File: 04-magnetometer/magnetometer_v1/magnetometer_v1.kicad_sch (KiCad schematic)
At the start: 42 parts, among them IC1 STM32F072CBT6, IC2 TMAG5170A1QDGKR, IC3 TCAN1042GVDRQ1, J1 Conn_02x04_Odd_Even, J2 USB4110-GF-A, SW3 SW_SPDT, U1 SPX3819M5-L-3-3/TR, U2 NANOT100AS, U3 NANOT100AS

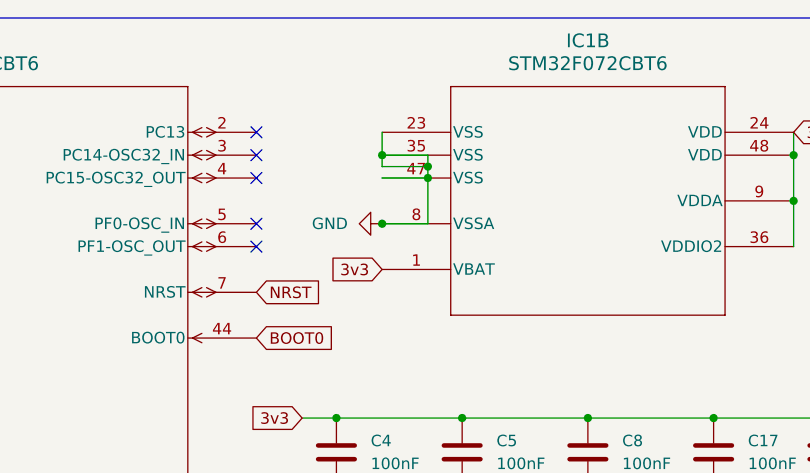
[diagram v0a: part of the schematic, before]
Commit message: made review changes
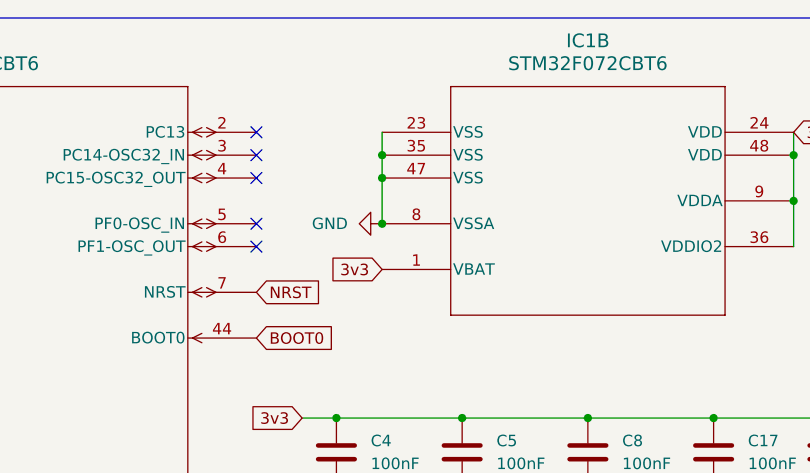
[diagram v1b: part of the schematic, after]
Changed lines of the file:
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@@
 	)
 	(junction
-		(at 114.3 33.02)
+		(at 109.22 34.29)
 		(diameter 0)
 		(color 0 0 0 0)
@@
 	)
 	(junction
-		(at 114.3 34.29)
-		(diameter 0)
-		(color 0 0 0 0)
-	)
-	(junction
 		(at 113.03 151.13)
 		(diameter 0)
@@
 	(wire
 		(pts
-			(xy 109.22 33.02) (xy 114.3 33.02)
-		)
-		(stroke
-			(width 0)
-			(type default)
-		)
-	)
-	(wire
-		(pts
 			(xy 143.51 118.11) (xy 143.51 119.38)
 		)
@@
 	(wire
 		(pts
-			(xy 114.3 33.02) (xy 114.3 34.29)
-		)
-		(stroke
-			(width 0)
-			(type default)
-		)
-	)
-	(wire
-		(pts
 			(xy 104.14 78.74) (xy 118.11 78.74)
 		)
@@
 	(wire
 		(pts
-			(xy 114.3 33.02) (xy 114.3 31.75)
-		)
-		(stroke
-			(width 0)
-			(type default)
-		)
-	)
-	(wire
-		(pts
 			(xy 251.46 118.11) (xy 248.92 118.11)
 		)
@@
 	(wire
 		(pts
-			(xy 109.22 34.29) (xy 114.3 34.29)
-		)
-		(stroke
-			(width 0)
-			(type default)
-		)
-	)
-	(wire
-		(pts
 			(xy 248.92 114.3) (xy 259.08 114.3)
 		)
@@
 	(wire
 		(pts
-			(xy 109.22 31.75) (xy 109.22 33.02)
+			(xy 109.22 31.75) (xy 109.22 34.29)
 		)
 		(stroke
@@
 	(wire
 		(pts
-			(xy 109.22 39.37) (xy 114.3 39.37)
-		)
-		(stroke
-			(width 0)
-			(type default)
-		)
-	)
-	(wire
-		(pts
 			(xy 215.9 142.24) (xy 215.9 147.32)
 		)
@@
 	(wire
 		(pts
-			(xy 114.3 34.29) (xy 114.3 39.37)
-		)
-		(stroke
-			(width 0)
-			(type default)
-		)
-	)
-	(wire
-		(pts
-			(xy 109.22 31.75) (xy 114.3 31.75)
-		)
-		(stroke
+			(xy 109.22 34.29) (xy 109.22 39.37)
+		)
+		(stroke
